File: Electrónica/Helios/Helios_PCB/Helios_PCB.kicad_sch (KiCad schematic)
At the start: 18 parts, among them Q1 AO3400A

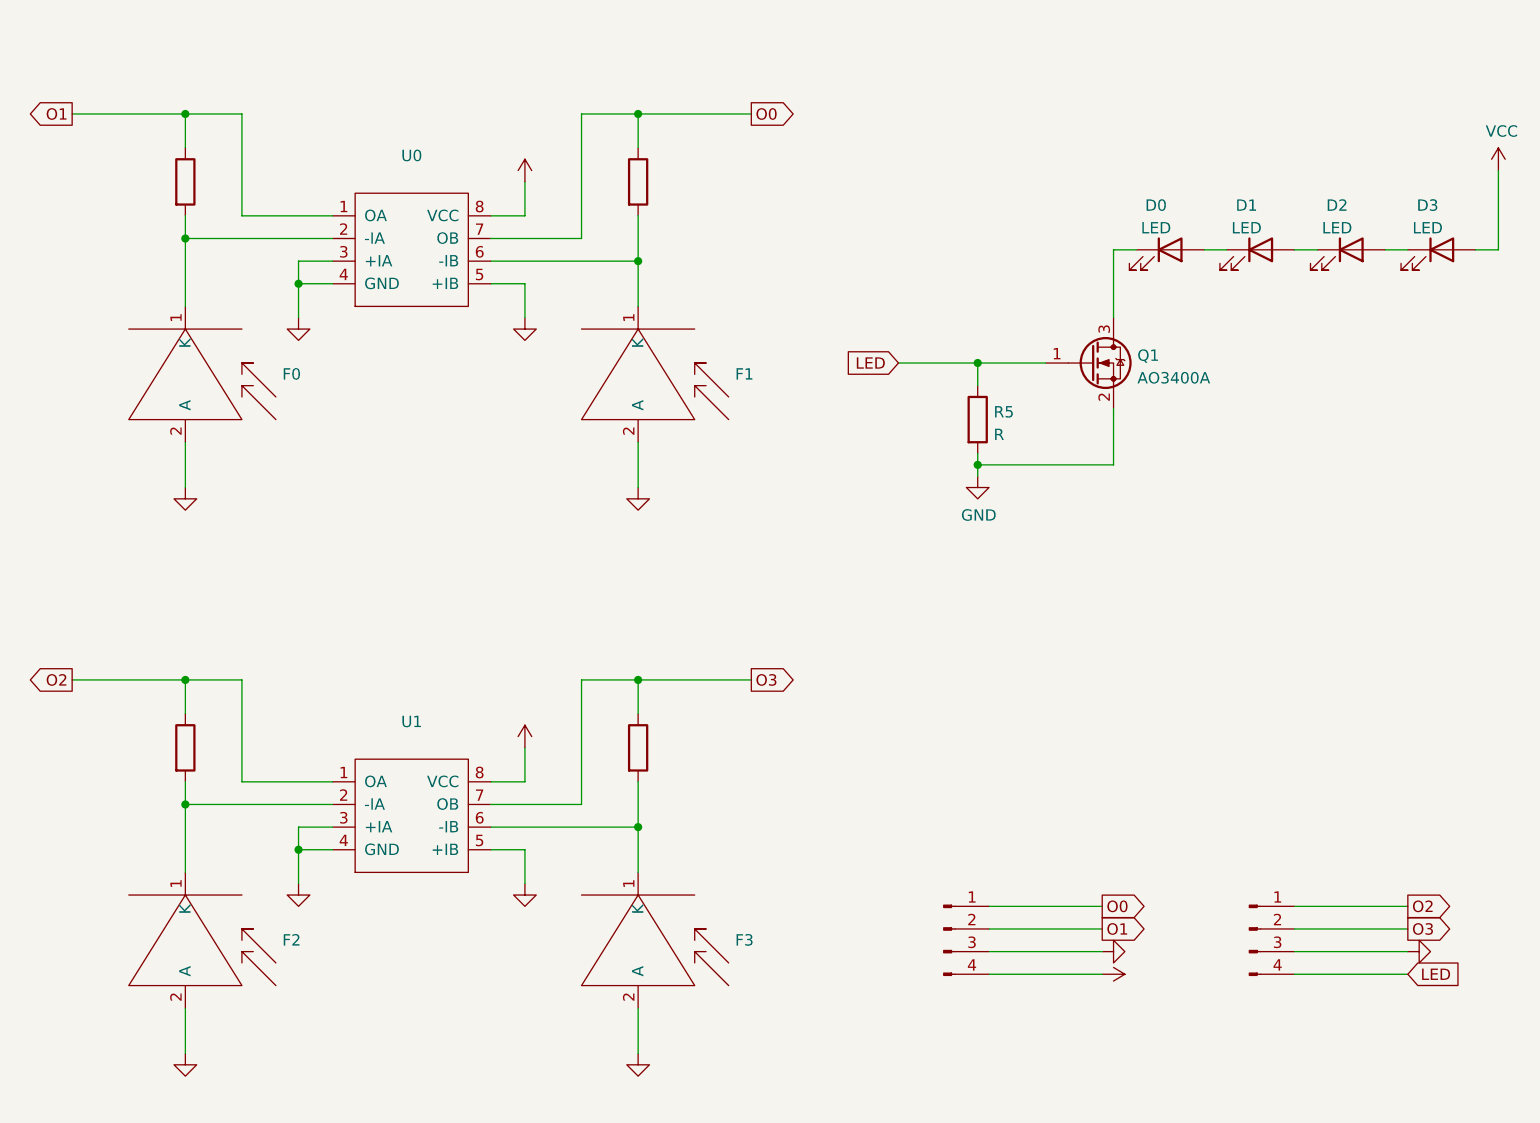
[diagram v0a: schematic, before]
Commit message: Revert "Revert "Helios: Bot added resistance""
This reverts commit b6ec3ea842d96de8bcfcf6a4a844077dd7699937.
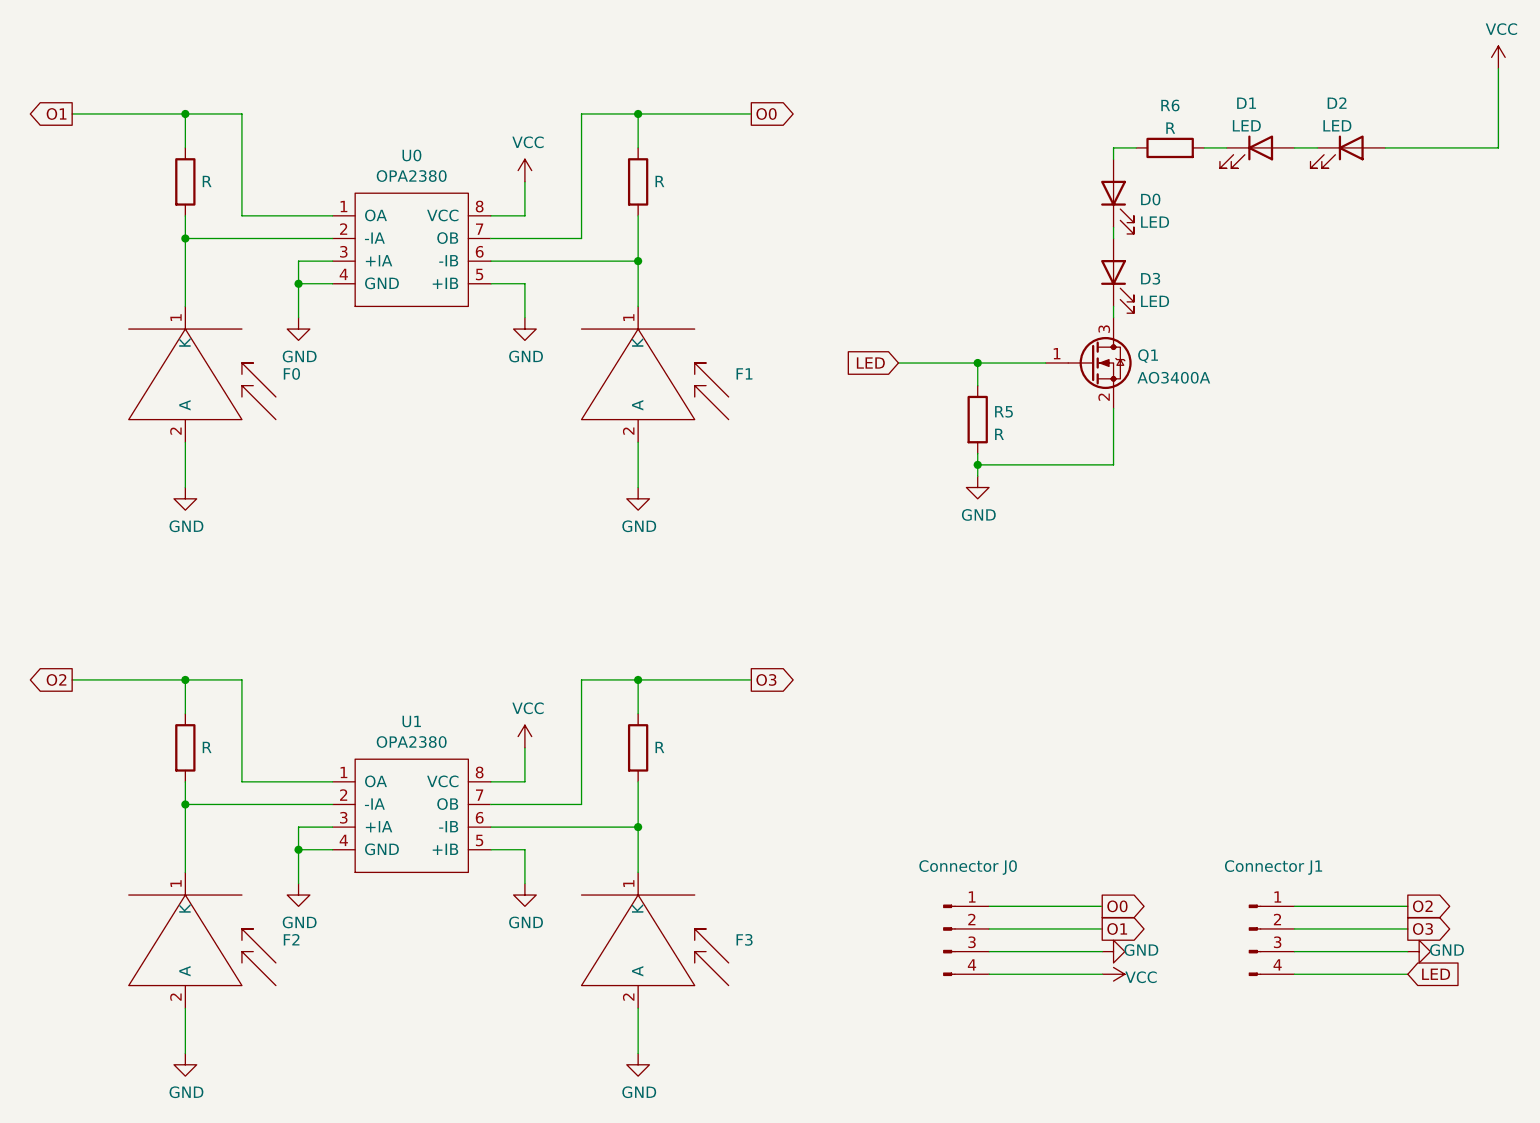
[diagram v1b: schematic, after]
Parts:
- added R6: R, Helios:RS_0805, symbol Device:R
- F0, F1, F2, F3: value (none) -> SFH2704; footprint (none) -> Helios:SFH2704_Photodiode
- J0: value (none) -> Connector J0; footprint (none) -> Connector_PinHeader_2.00mm:PinHeader_1x04_P2.00mm_Vertical
- J1: value (none) -> Connector J1; footprint (none) -> Connector_PinHeader_2.00mm:PinHeader_1x04_P2.00mm_Vertical
- R0, R1, R2, R3: value (none) -> R; footprint (none) -> Helios:RS_0805
- U0, U1: value (none) -> OPA2380; footprint (none) -> Helios:OPA2380
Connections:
- net VCC: now also D2.2 (A); no longer D3.2 (A)
- net at D1.1 (K): now also R6.2; no longer D0.2 (A)
- net at D3.1 (K): now also Q1.3 (D); no longer D2.2 (A)
- net at D0.1 (K): now also D3.2 (A); no longer Q1.3 (D)
- new net: D0.2 (A), R6.1
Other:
- moved on the sheet: D0, D1, D2, D3

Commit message: Revert "Helios: Bot added resistance"
This reverts commit d0f403256e0d7f179b5c0dd237f6584baac4939d.
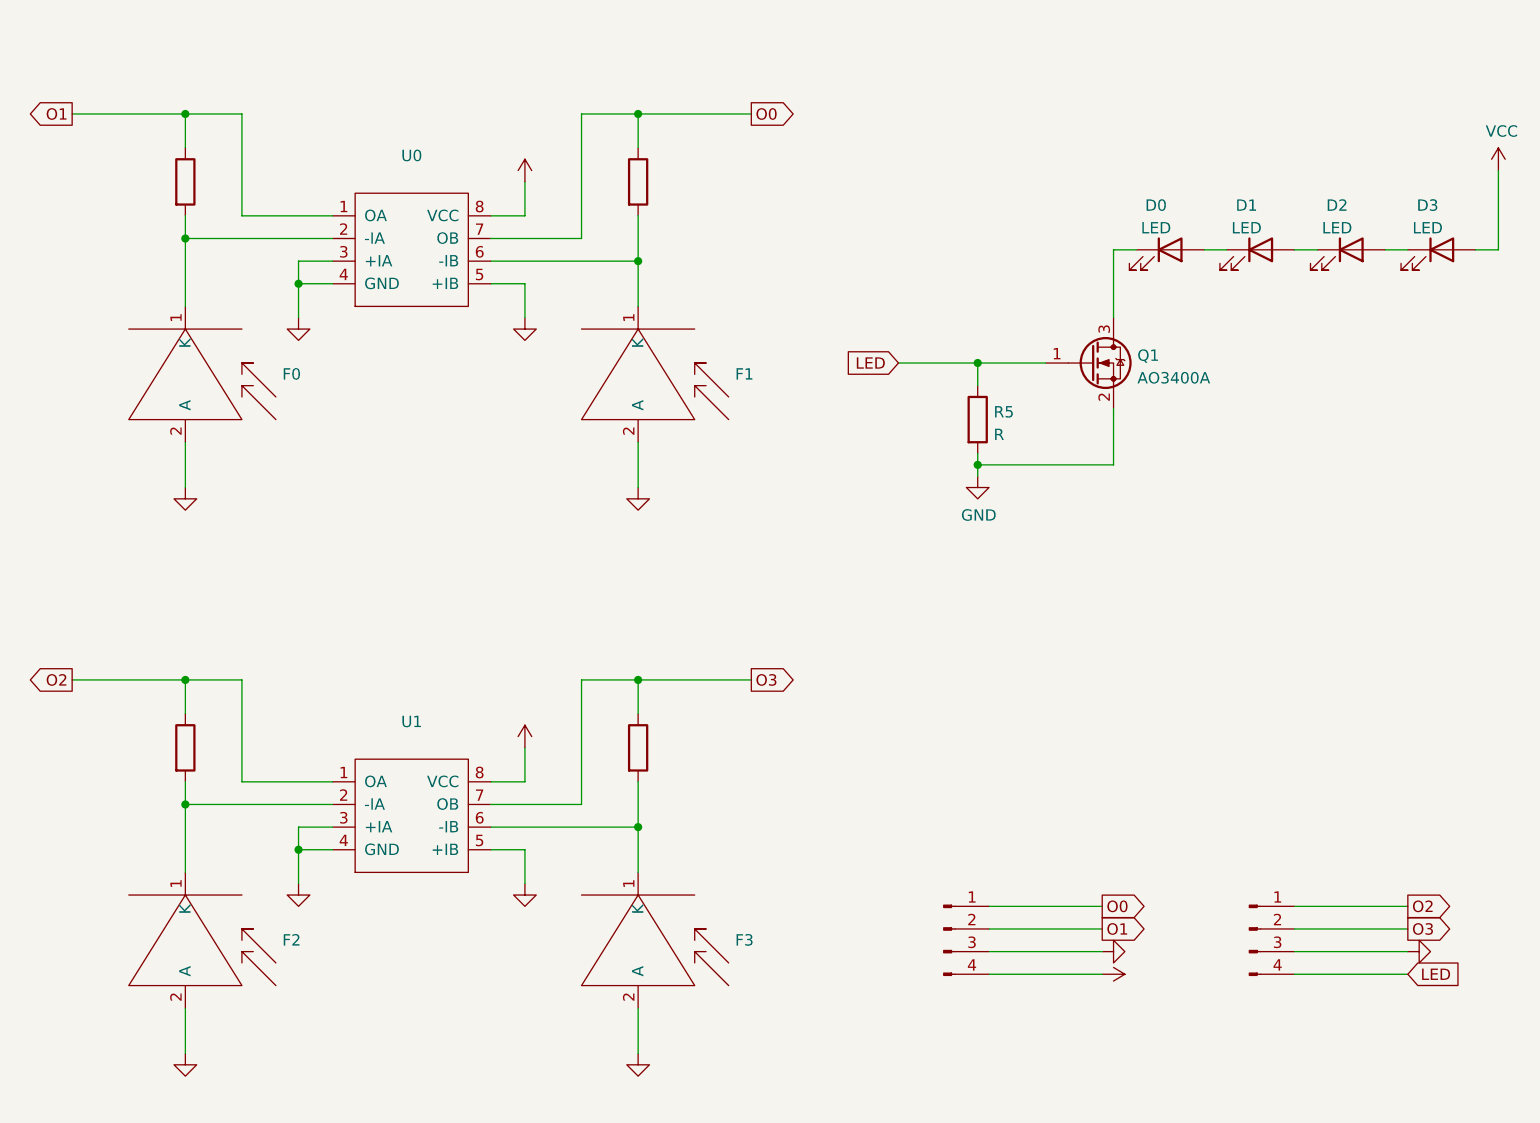
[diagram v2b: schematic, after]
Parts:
- removed R6: R, Helios:RS_0805, symbol Device:R
- F0, F1, F2, F3: value SFH2704 -> (none); footprint Helios:SFH2704_Photodiode -> (none)
- J0: value Connector J0 -> (none); footprint Connector_PinHeader_2.00mm:PinHeader_1x04_P2.00mm_Vertical -> (none)
- J1: value Connector J1 -> (none); footprint Connector_PinHeader_2.00mm:PinHeader_1x04_P2.00mm_Vertical -> (none)
- R0, R1, R2, R3: value R -> (none); footprint Helios:RS_0805 -> (none)
- U0, U1: value OPA2380 -> (none); footprint Helios:OPA2380 -> (none)
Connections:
- net VCC: now also D3.2 (A); no longer D2.2 (A)
- net at D1.1 (K): now also D0.2 (A)
- net at D3.1 (K): now also D2.2 (A); no longer Q1.3 (D)
- net at D0.1 (K): now also Q1.3 (D); no longer D3.2 (A)
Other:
- moved on the sheet: D0, D1, D2, D3
